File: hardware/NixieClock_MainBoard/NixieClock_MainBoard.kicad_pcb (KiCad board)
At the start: 2 copper layers, 152.4 x 63.5 mm, 106 parts, among them J1 Conn_01x14, J10 Conn_01x04, J11 Conn_01x04, J12 Conn_01x03, J13 Conn_01x03, J2 Conn_01x08, J3 Conn_01x08, J4 Conn_01x08, J5 Conn_01x08, J6 USB_C_Receptacle_USB2.0_16P, J7 Micro_SD_Card, J8 Conn_01x08, J9 Conn_01x03, Q1 BC847, Q2 BC847, Q3 Si4532DY, U1 ESP32-WROOM-32E, U10 NC7SZ125M5X, U12 NC7SZ125M5X, U13 NC7SZ125M5X, U14 CP2102N-Axx-xQFN24, U15 CH340C, U16 NC7SZ125M5X, U17 NC7SZ125M5X, U18 NC7SZ125M5X, U19 NC7SZ125M5X, U2 R-78C3.3-1.0, U20 NC7SZ125M5X, U21 NC7SZ125M5X, U3 NC7SZ125M5X, U4 PCA9635, U5 NC7SZ125M5X, U6 PCA9538A, U7 NC7SZ125M5X, U8 NC7SZ125M5X, U9 NC7SZ125M5X

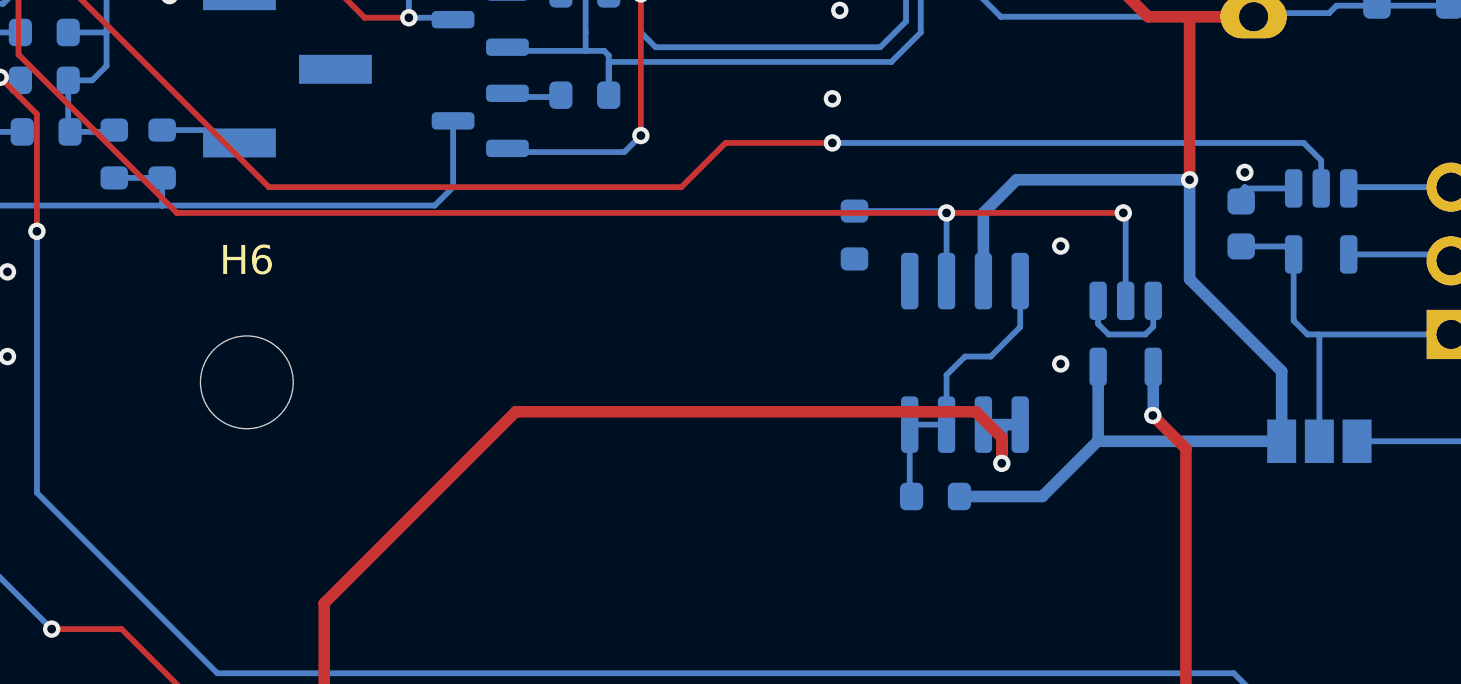
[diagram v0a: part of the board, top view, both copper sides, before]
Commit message: Version 2 Ready
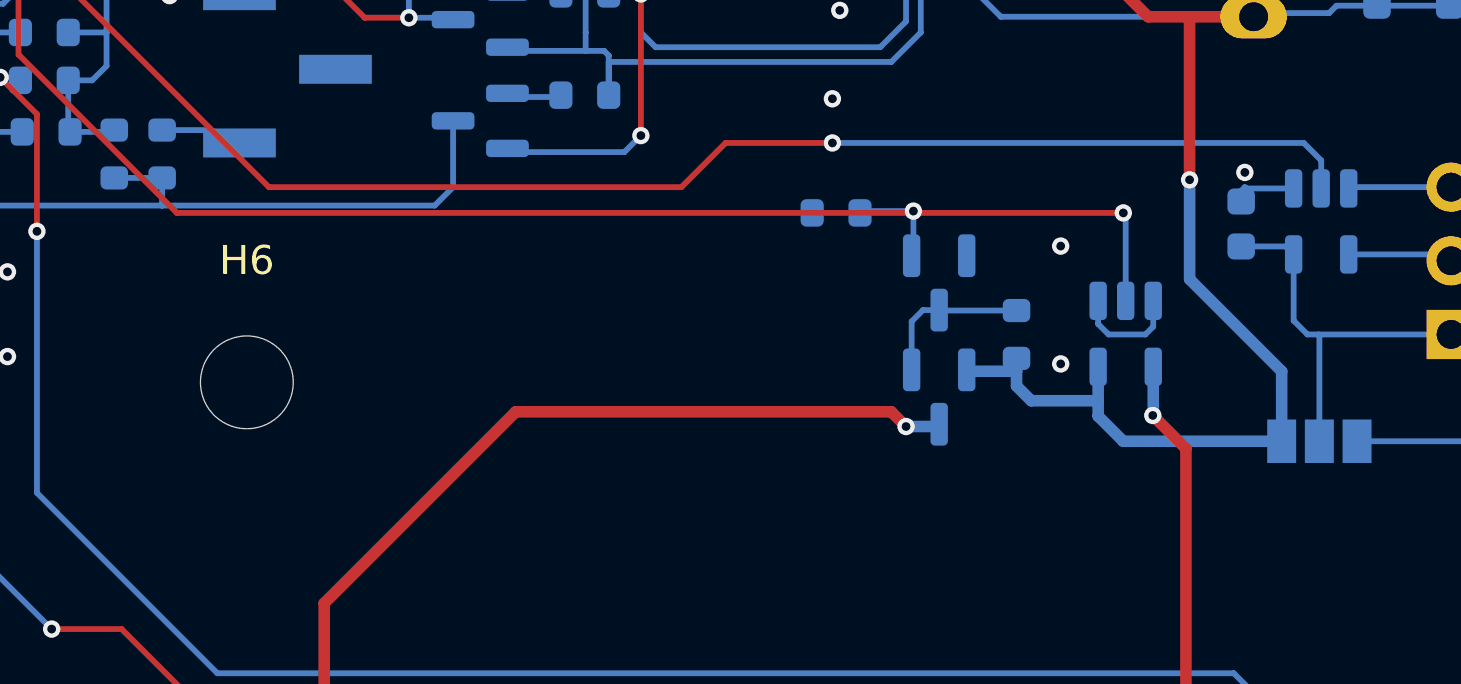
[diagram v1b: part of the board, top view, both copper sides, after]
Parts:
- added Q4: Si2319CDS, Package_TO_SOT_SMD:SOT-23, B.Cu at (169.3, 110.0)
- Q3: value Si4532DY -> BSS123; footprint Package_SO:SOIC-8_3.9x4.9mm_P1.27mm -> Package_TO_SOT_SMD:SOT-23
- R28, R30: value 10k -> 470R
- moved R34 6.25 mm to (172.0, 107.8), turned to 90 degrees
- moved Q3 2.57 mm to (169.3, 106.0)
- moved R33 0.99 mm to (165.7, 103.6), turned to 180 degrees
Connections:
- Q3 pad 1: GND -> /DISP_POWER_EN
- Q3 pad 2: /DISP_POWER_EN -> GND
- Q3 pad 3: +3.3V -> Net-(Q3-D)
- R34 pad 2: Net-(Q3B-G) -> Net-(Q3-D)
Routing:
- net +3.3V: track 489.6 -> 479.3 mm
- net Net-(Q3B-G): track 10.3 -> 0.00 mm
- net /VDD: track 181.9 -> 176.1 mm
- net Net-(Q3-D): track 0.00 -> 5.45 mm
- net /DISP_POWER_EN: track 55.2 -> 53.3 mm
